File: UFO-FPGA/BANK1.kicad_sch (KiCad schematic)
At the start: 3 parts, among them U4 ICE40HX4K-TQ144

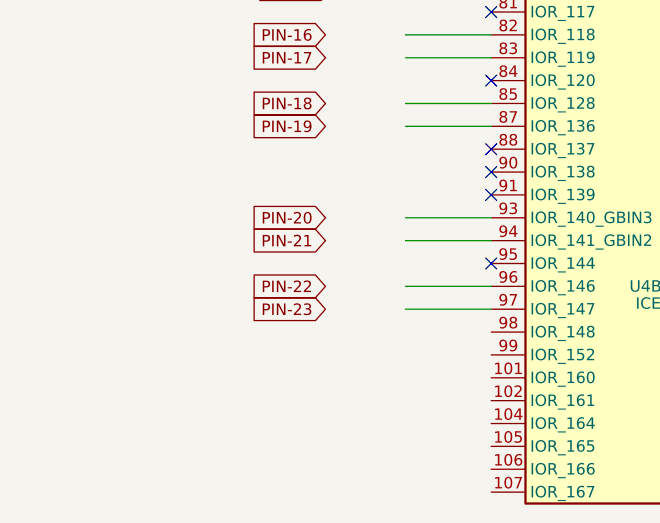
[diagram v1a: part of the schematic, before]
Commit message: pcb
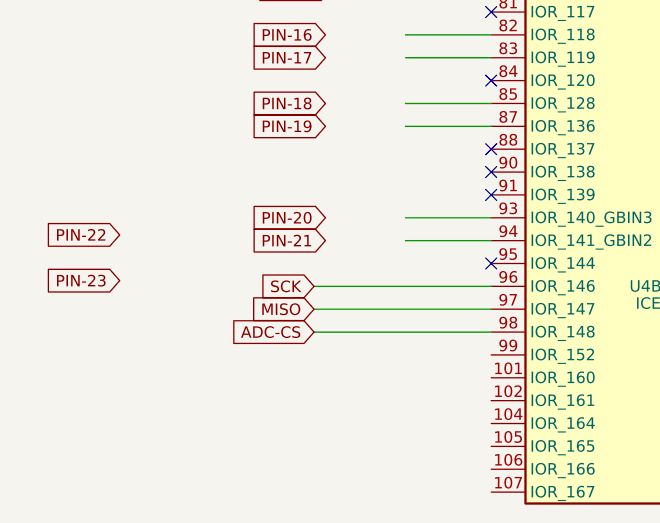
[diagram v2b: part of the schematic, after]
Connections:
- net SCK: now reaches U4.96 (IOR_146)
- net MISO: now reaches U4.97 (IOR_147)
- net ADC-CS: now reaches U4.98 (IOR_148)
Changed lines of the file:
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@@
     (stroke (width 0) (type default))
   )
-  (wire (pts (xy 116.205 120.65) (xy 125.73 120.65))
+  (wire (pts (xy 106.045 120.65) (xy 125.73 120.65))
     (stroke (width 0) (type default))
   )
@@
     (stroke (width 0) (type default))
   )
+  (wire (pts (xy 106.045 125.73) (xy 125.73 125.73))
+    (stroke (width 0) (type default))
+  )
   (wire (pts (xy 116.205 95.25) (xy 125.73 95.25))
     (stroke (width 0) (type default))
@@
     (stroke (width 0) (type default))
   )
-  (wire (pts (xy 116.205 123.19) (xy 125.73 123.19))
+  (wire (pts (xy 106.045 123.19) (xy 125.73 123.19))
     (stroke (width 0) (type default))
   )
@@
     (effects (font (size 1.27 1.27)) (justify left bottom))
   )
-  (global_label "PIN-23" (shape input) (at 107.315 123.19 180) (fields_autoplaced)
+  (global_label "MISO" (shape input) (at 106.045 123.19 180) (fields_autoplaced)
     (effects (font (size 1.27 1.27)) (justify right))
-    (property "Intersheetrefs" "${INTERSHEET_REFS}" (at 97.2125 123.19 0)
+    (property "Intersheetrefs" "${INTERSHEET_REFS}" (at 98.543 123.19 0)
+      (effects (font (size 1.27 1.27)) (justify right) hide)
+    )
+  )
+  (global_label "PIN-23" (shape input) (at 84.455 120.015 180) (fields_autoplaced)
+    (effects (font (size 1.27 1.27)) (justify right))
+    (property "Intersheetrefs" "${INTERSHEET_REFS}" (at 74.3525 120.015 0)
       (effects (font (size 1.27 1.27)) (justify right) hide)
     )
@@
     (effects (font (size 1.27 1.27)) (justify right))
     (property "Intersheetrefs" "${INTERSHEET_REFS}" (at 97.8475 72.39 0)
+      (effects (font (size 1.27 1.27)) (justify right) hide)
+    )
+  )
+  (global_label "ADC-CS" (shape input) (at 106.045 125.73 180) (fields_autoplaced)
+    (effects (font (size 1.27 1.27)) (justify right))
+    (property "Intersheetrefs" "${INTERSHEET_REFS}" (at 95.4587 125.73 0)
+      (effects (font (size 1.27 1.27)) (justify right) hide)
+    )
+  )
+  (global_label "SCK" (shape input) (at 106.045 120.65 180) (fields_autoplaced)
+    (effects (font (size 1.27 1.27)) (justify right))
+    (property "Intersheetrefs" "${INTERSHEET_REFS}" (at 99.3897 120.65 0)
       (effects (font (size 1.27 1.27)) (justify right) hide)
     )
@@
     )
   )
-  (global_label "PIN-22" (shape input) (at 107.315 120.65 180) (fields_autoplaced)
+  (global_label "PIN-22" (shape input) (at 84.455 114.935 180) (fields_autoplaced)
     (effects (font (size 1.27 1.27)) (justify right))
-    (property "Intersheetrefs" "${INTERSHEET_REFS}" (at 97.2125 120.65 0)
+    (property "Intersheetrefs" "${INTERSHEET_REFS}" (at 74.3525 114.935 0)
       (effects (font (size 1.27 1.27)) (justify right) hide)
     )

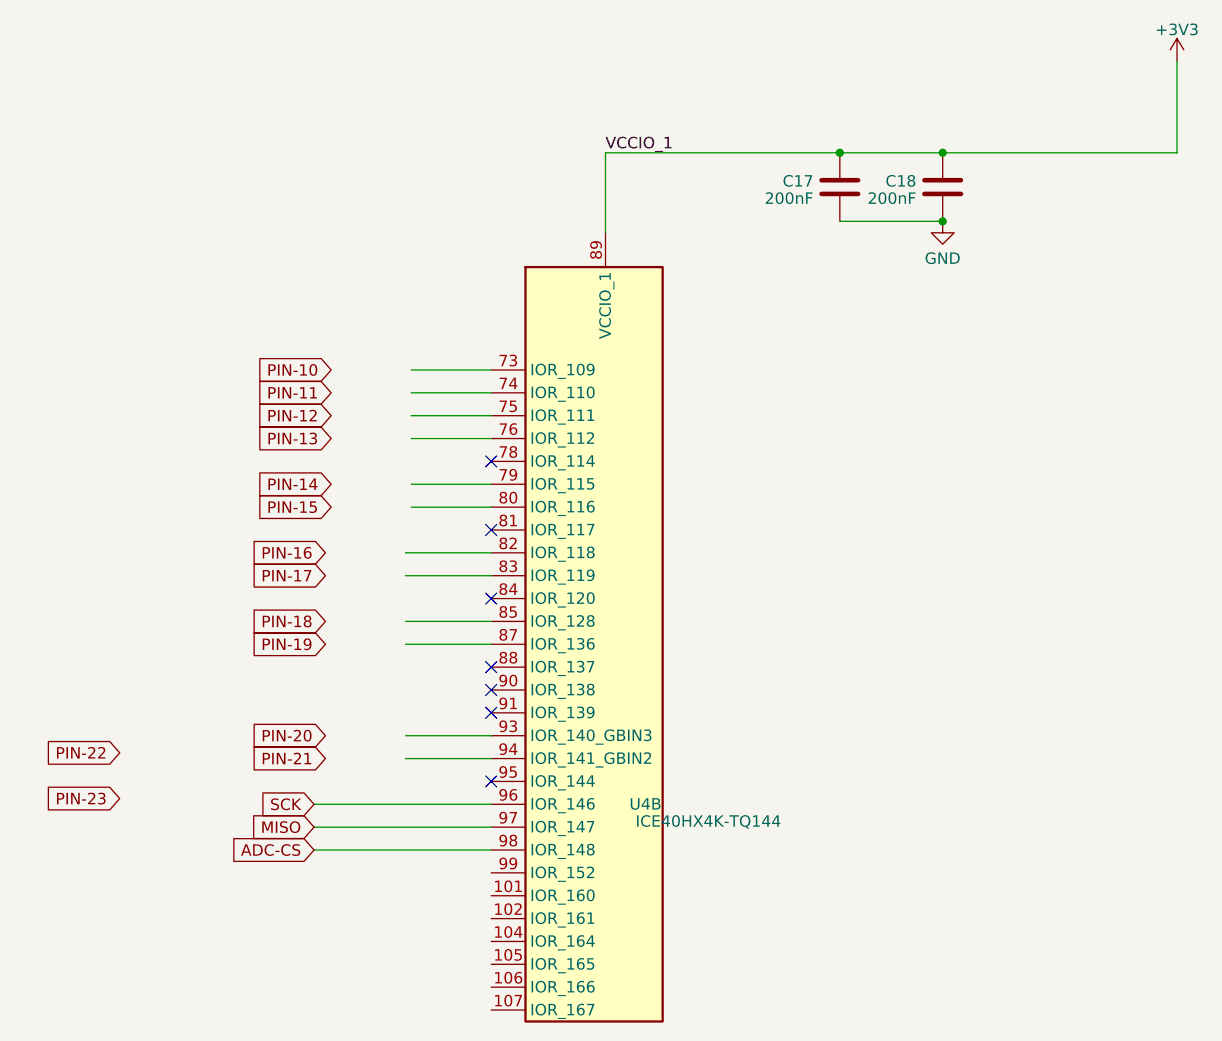
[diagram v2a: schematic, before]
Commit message: pcb
added monkey
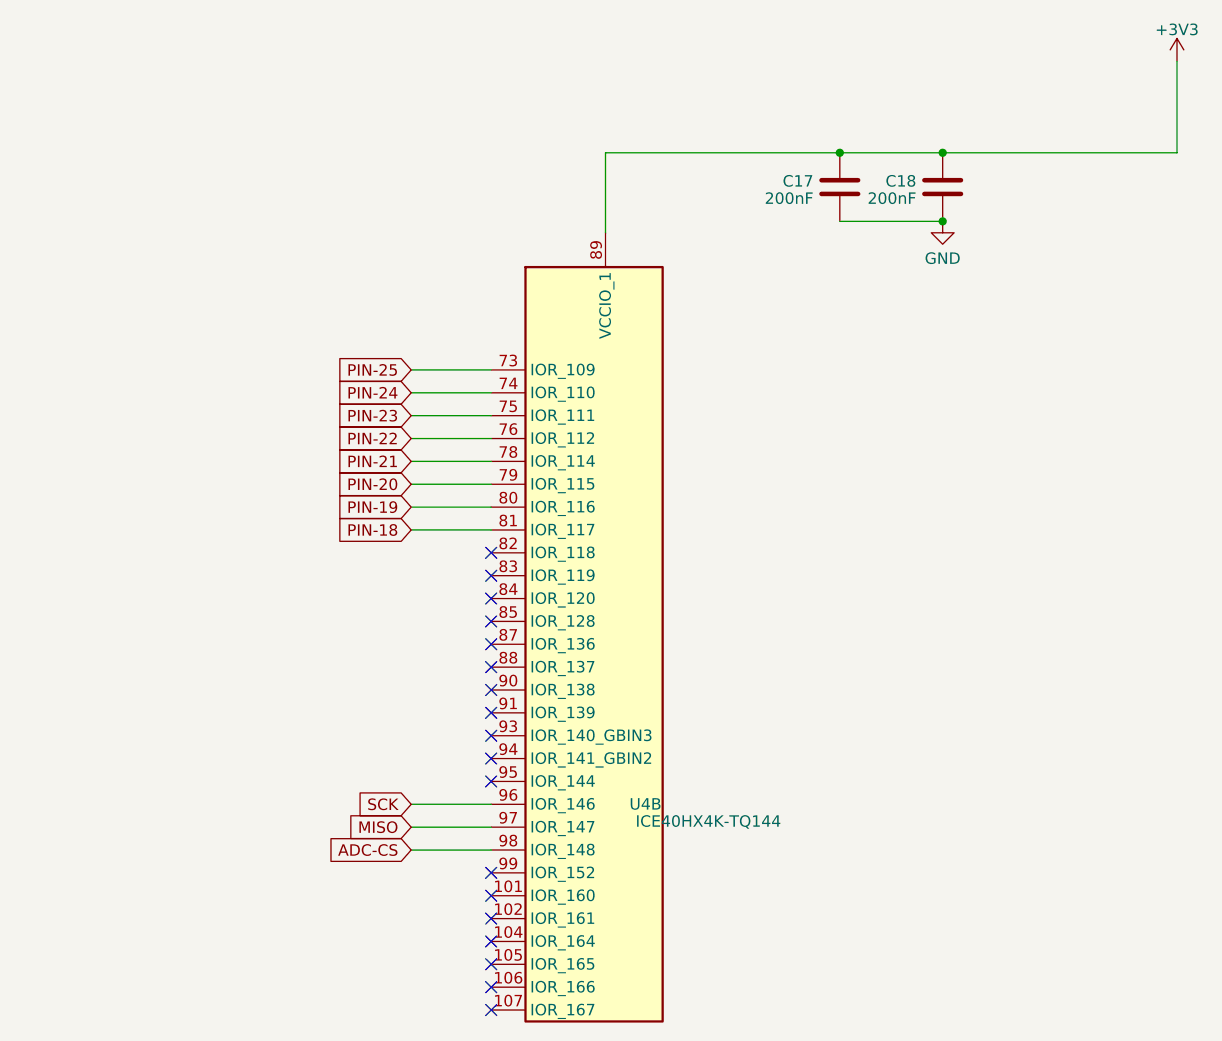
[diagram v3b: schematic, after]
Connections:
- net PIN-18: now also U4.81 (IOR_117)
- net PIN-19: now also U4.80 (IOR_116)
- net PIN-20: now also U4.79 (IOR_115)
- net PIN-21: now also U4.78 (IOR_114)
- net PIN-22: now also U4.76 (IOR_112)
- net PIN-23: now also U4.75 (IOR_111)
- net PIN-25: now reaches U4.73 (IOR_109)
- net PIN-24: now reaches U4.74 (IOR_110)
- no-connect marks 7 -> 18
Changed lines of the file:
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@@
   )
   (no_connect (at 125.73 118.11))
-  (no_connect (at 125.73 82.55))
+  (no_connect (at 125.73 138.43))
   (no_connect (at 125.73 105.41))
+  (no_connect (at 125.73 92.71))
   (no_connect (at 125.73 97.79))
-  (no_connect (at 125.73 90.17))
+  (no_connect (at 125.73 143.51))
+  (no_connect (at 125.73 140.97))
+  (no_connect (at 125.73 130.81))
+  (no_connect (at 125.73 135.89))
+  (no_connect (at 125.73 95.25))
+  (no_connect (at 125.73 100.33))
+  (no_connect (at 125.73 133.35))
+  (no_connect (at 125.73 113.03))
   (no_connect (at 125.73 110.49))
+  (no_connect (at 125.73 128.27))
+  (no_connect (at 125.73 115.57))
   (no_connect (at 125.73 107.95))
+  (no_connect (at 125.73 102.87))
   (wire (pts (xy 116.84 80.01) (xy 125.73 80.01))
     (stroke (width 0) (type default))
@@
     (stroke (width 0) (type default))
   )
-  (wire (pts (xy 106.045 120.65) (xy 125.73 120.65))
-    (stroke (width 0) (type default))
-  )
   (wire (pts (xy 116.84 77.47) (xy 125.73 77.47))
-    (stroke (width 0) (type default))
-  )
-  (wire (pts (xy 116.205 113.03) (xy 125.73 113.03))
     (stroke (width 0) (type default))
   )
@@
     (stroke (width 0) (type default))
   )
-  (wire (pts (xy 106.045 125.73) (xy 125.73 125.73))
-    (stroke (width 0) (type default))
-  )
-  (wire (pts (xy 116.205 95.25) (xy 125.73 95.25))
+  (wire (pts (xy 116.84 90.17) (xy 125.73 90.17))
     (stroke (width 0) (type default))
   )
@@
     (stroke (width 0) (type default))
   )
-  (wire (pts (xy 116.205 92.71) (xy 125.73 92.71))
+  (wire (pts (xy 116.84 82.55) (xy 125.73 82.55))
     (stroke (width 0) (type default))
   )
@@
     (stroke (width 0) (type default))
   )
-  (wire (pts (xy 106.045 123.19) (xy 125.73 123.19))
+  (wire (pts (xy 116.84 123.19) (xy 125.73 123.19))
     (stroke (width 0) (type default))
   )
-  (wire (pts (xy 116.205 102.87) (xy 125.73 102.87))
+  (wire (pts (xy 116.84 120.65) (xy 125.73 120.65))
     (stroke (width 0) (type default))
   )
-  (wire (pts (xy 116.205 115.57) (xy 125.73 115.57))
+  (wire (pts (xy 116.84 125.73) (xy 125.73 125.73))
     (stroke (width 0) (type default))
   )
@@
     (stroke (width 0) (type default))
   )
-  (wire (pts (xy 116.205 100.33) (xy 125.73 100.33))
-    (stroke (width 0) (type default))
-  )
   (wire (pts (xy 164.465 55.88) (xy 175.895 55.88))
     (stroke (width 0) (type default))
   )
-  (label "VCCIO_1" (at 138.43 48.26 0) (fields_autoplaced)
-    (effects (font (size 1.27 1.27)) (justify left bottom))
-  )
-  (global_label "MISO" (shape input) (at 106.045 123.19 180) (fields_autoplaced)
+  (global_label "MISO" (shape input) (at 116.84 123.19 180) (fields_autoplaced)
     (effects (font (size 1.27 1.27)) (justify right))
-    (property "Intersheetrefs" "${INTERSHEET_REFS}" (at 98.543 123.19 0)
+    (property "Intersheetrefs" "${INTERSHEET_REFS}" (at 109.338 123.19 0)
       (effects (font (size 1.27 1.27)) (justify right) hide)
     )
   )
-  (global_label "PIN-23" (shape input) (at 84.455 120.015 180) (fields_autoplaced)
+  (global_label "PIN-23" (shape input) (at 116.84 77.47 180) (fields_autoplaced)
     (effects (font (size 1.27 1.27)) (justify right))
-    (property "Intersheetrefs" "${INTERSHEET_REFS}" (at 74.3525 120.015 0)
+    (property "Intersheetrefs" "${INTERSHEET_REFS}" (at 106.7375 77.47 0)
       (effects (font (size 1.27 1.27)) (justify right) hide)
     )
   )
-  (global_label "PIN-10" (shape input) (at 107.95 72.39 180) (fields_autoplaced)
+  (global_label "PIN-18" (shape input) (at 116.84 90.17 180) (fields_autoplaced)
     (effects (font (size 1.27 1.27)) (justify right))
-    (property "Intersheetrefs" "${INTERSHEET_REFS}" (at 97.8475 72.39 0)
+    (property "Intersheetrefs" "${INTERSHEET_REFS}" (at 106.7375 90.17 0)
       (effects (font (size 1.27 1.27)) (justify right) hide)
     )
   )
-  (global_label "ADC-CS" (shape input) (at 106.045 125.73 180) (fields_autoplaced)
+  (global_label "ADC-CS" (shape input) (at 116.84 125.73 180) (fields_autoplaced)
     (effects (font (size 1.27 1.27)) (justify right))
-    (property "Intersheetrefs" "${INTERSHEET_REFS}" (at 95.4587 125.73 0)
+    (property "Intersheetrefs" "${INTERSHEET_REFS}" (at 106.2537 125.73 0)
       (effects (font (size 1.27 1.27)) (justify right) hide)
     )
   )
-  (global_label "SCK" (shape input) (at 106.045 120.65 180) (fields_autoplaced)
+  (global_label "SCK" (shape input) (at 116.84 120.65 180) (fields_autoplaced)
     (effects (font (size 1.27 1.27)) (justify right))
-    (property "Intersheetrefs" "${INTERSHEET_REFS}" (at 99.3897 120.65 0)
+    (property "Intersheetrefs" "${INTERSHEET_REFS}" (at 110.1847 120.65 0)
       (effects (font (size 1.27 1.27)) (justify right) hide)
     )
   )
-  (global_label "PIN-16" (shape input) (at 107.315 92.71 180) (fields_autoplaced)
+  (global_label "PIN-21" (shape input) (at 116.84 82.55 180) (fields_autoplaced)
     (effects (font (size 1.27 1.27)) (justify right))
-    (property "Intersheetrefs" "${INTERSHEET_REFS}" (at 97.2125 92.71 0)
+    (property "Intersheetrefs" "${INTERSHEET_REFS}" (at 106.7375 82.55 0)
       (effects (font (size 1.27 1.27)) (justify right) hide)
     )
   )
-  (global_label "PIN-13" (shape input) (at 107.95 80.01 180) (fields_autoplaced)
+  (global_label "PIN-20" (shape input) (at 116.84 85.09 180) (fields_autoplaced)
     (effects (font (size 1.27 1.27)) (justify right))
-    (property "Intersheetrefs" "${INTERSHEET_REFS}" (at 97.8475 80.01 0)
+    (property "Intersheetrefs" "${INTERSHEET_REFS}" (at 106.7375 85.09 0)
       (effects (font (size 1.27 1.27)) (justify right) hide)
     )
   )
-  (global_label "PIN-18" (shape input) (at 107.315 100.33 180) (fields_autoplaced)
+  (global_label "PIN-22" (shape input) (at 116.84 80.01 180) (fields_autoplaced)
     (effects (font (size 1.27 1.27)) (justify right))
-    (property "Intersheetrefs" "${INTERSHEET_REFS}" (at 97.2125 100.33 0)
+    (property "Intersheetrefs" "${INTERSHEET_REFS}" (at 106.7375 80.01 0)
       (effects (font (size 1.27 1.27)) (justify right) hide)
     )
   )
-  (global_label "PIN-22" (shape input) (at 84.455 114.935 180) (fields_autoplaced)
+  (global_label "PIN-19" (shape input) (at 116.84 87.63 180) (fields_autoplaced)
     (effects (font (size 1.27 1.27)) (justify right))
-    (property "Intersheetrefs" "${INTERSHEET_REFS}" (at 74.3525 114.935 0)
+    (property "Intersheetrefs" "${INTERSHEET_REFS}" (at 106.7375 87.63 0)
       (effects (font (size 1.27 1.27)) (justify right) hide)
     )
   )
-  (global_label "PIN-19" (shape input) (at 107.315 102.87 180) (fields_autoplaced)
+  (global_label "PIN-25" (shape input) (at 116.84 72.39 180) (fields_autoplaced)
     (effects (font (size 1.27 1.27)) (justify right))
-    (property "Intersheetrefs" "${INTERSHEET_REFS}" (at 97.2125 102.87 0)
+    (property "Intersheetrefs" "${INTERSHEET_REFS}" (at 106.7375 72.39 0)
       (effects (font (size 1.27 1.27)) (justify right) hide)
     )
   )
-  (global_label "PIN-11" (shape input) (at 107.95 74.93 180) (fields_autoplaced)
+  (global_label "PIN-24" (shape input) (at 116.84 74.93 180) (fields_autoplaced)
     (effects (font (size 1.27 1.27)) (justify right))
-    (property "Intersheetrefs" "${INTERSHEET_REFS}" (at 97.8475 74.93 0)
+    (property "Intersheetrefs" "${INTERSHEET_REFS}" (at 106.7375 74.93 0)
       (effects (font (size 1.27 1.27)) (justify right) hide)
     )
-  )
-  (global_label "PIN-20" (shape input) (at 107.315 113.03 180) (fields_autoplaced)
-    (effects (font (size 1.27 1.27)) (justify right))
-    (property "Intersheetrefs" "${INTERSHEET_REFS}" (at 97.2125 113.03 0)
-      (effects (font (size 1.27 1.27)) (justify right) hide)
-    )
-  )
-  (global_label "PIN-12" (shape input) (at 107.95 77.47 180) (fields_autoplaced)
-    (effects (font (size 1.27 1.27)) (justify right))
-    (property "Intersheetrefs" "${INTERSHEET_REFS}" (at 97.8475 77.47 0)
-      (effects (font (size 1.27 1.27)) (justify right) hide)
-    )
-  )
-  (global_label "PIN-17" (shape input) (at 107.315 95.25 180) (fields_autoplaced)
-    (effects (font (size 1.27 1.27)) (justify right))
-    (property "Intersheetrefs" "${INTERSHEET_REFS}" (at 97.2125 95.25 0)
-      (effects (font (size 1.27 1.27)) (justify right) hide)
-    )
-  )
-  (global_label "PIN-15" (shape input) (at 107.95 87.63 180) (fields_autoplaced)
-    (effects (font (size 1.27 1.27)) (justify right))
-    (property "Intersheetrefs" "${INTERSHEET_REFS}" (at 97.8475 87.63 0)
-      (effects (font (size 1.27 1.27)) (justify right) hide)
-    )
-  )
-  (global_label "PIN-14" (shape input) (at 107.95 85.09 180) (fields_autoplaced)
-    (effects (font (size 1.27 1.27)) (justify right))
-    (property "Intersheetrefs" "${INTERSHEET_REFS}" (at 97.8475 85.09 0)
-      (effects (font (size 1.27 1.27)) (justify right) hide)
-    )
-  )
-  (global_label "PIN-21" (shape input) (at 107.315 115.57 180) (fields_autoplaced)
-    (effects (font (size 1.27 1.27)) (justify right))
-    (property "Intersheetrefs" "${INTERSHEET_REFS}" (at 97.2125 115.57 0)
-      (effects (font (size 1.27 1.27)) (justify right) hide)
-    )
